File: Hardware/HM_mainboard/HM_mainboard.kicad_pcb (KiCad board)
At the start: 2 copper layers, 80 x 55 mm, 58 parts, among them J1 JST PH2P ST90, J2 USB4105-GF-A, J3 Conn_01x04, J4 54-00174, J5 54-00174, J6 54-00174, J7 54-00174, Q1 PMOS - AS3401, U1 MCP73831-2, U2 TC1262-33, U3 ESP32-S3-WROOM-1, U4 WE-TVS-824015043, U5 MC6470, U6 BNO055, Y1 32.768 kHz

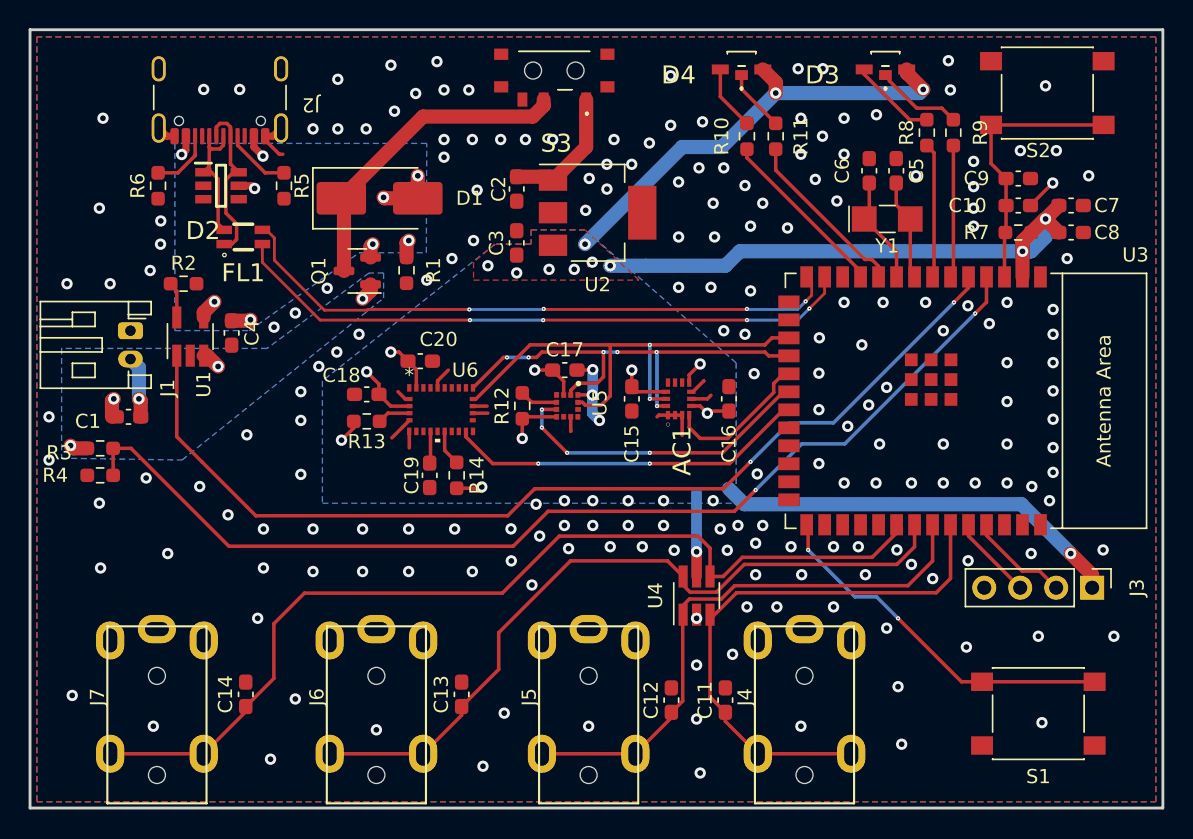
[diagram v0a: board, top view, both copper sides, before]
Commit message: Updated BOM
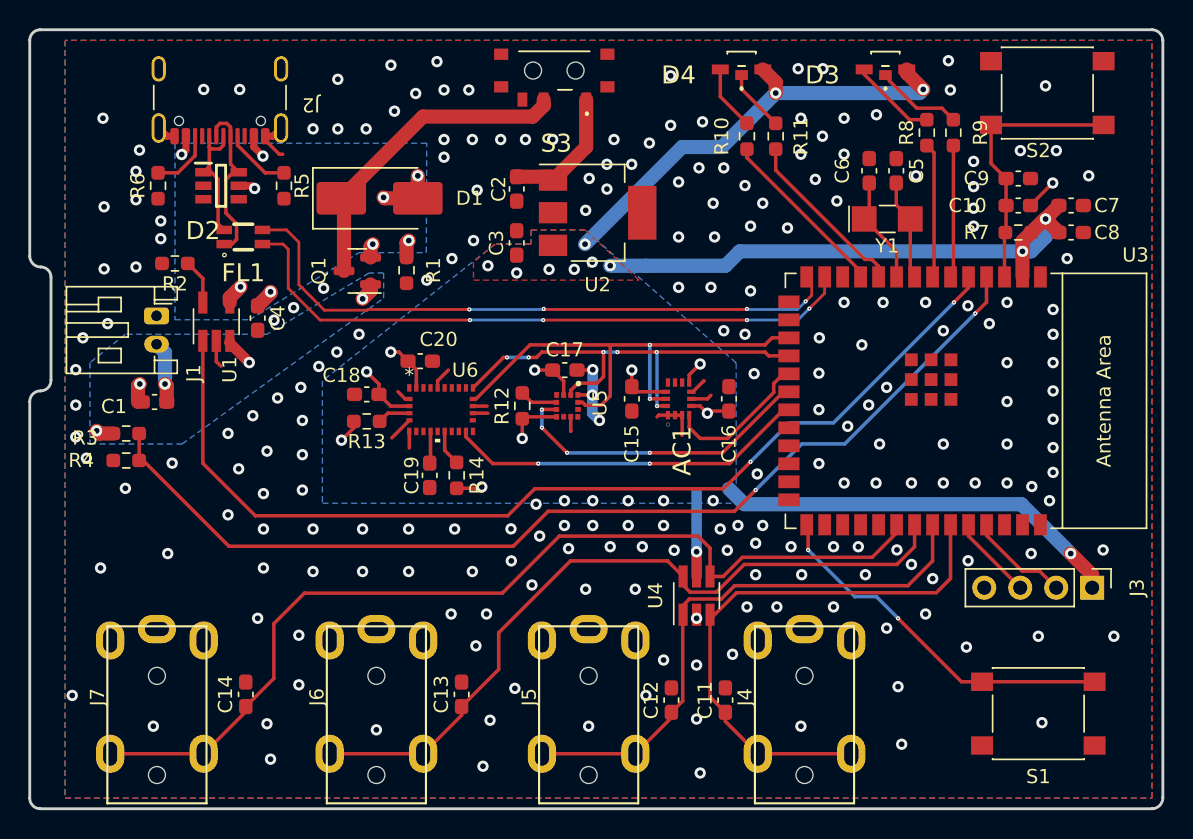
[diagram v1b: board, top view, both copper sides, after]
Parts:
- moved C4 2.12 mm to (132.8, 93.4)
- moved J1 2.12 mm to (125.7, 93.2)
- moved R3 2.12 mm to (123.6, 101.5)
- moved U1 2.12 mm to (129.9, 93.6)
- moved C1 2.12 mm to (125.6, 99.3)
- moved R4 2.12 mm to (123.6, 103.4)
- moved R2 1.56 mm to (127.0, 89.5), turned to 0 degrees
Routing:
- net /V_BATT_MEASURE: track 75.4 -> 73.2 mm
- net GND: track 28.7 -> 30.7 mm, vias 206 -> 228
- net Net-(U1-PROG): track 2.35 -> 3.20 mm
- net /Microcontroller - ESP32-S3-WROOM/USB_C_D-: track 44.6 -> 45.5 mm
- net /Microcontroller - ESP32-S3-WROOM/USB_C_D+: track 44.0 -> 44.8 mm
- net V_BATT: track 8.22 -> 9.00 mm
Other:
- outline, holes or cut-outs redrawn
